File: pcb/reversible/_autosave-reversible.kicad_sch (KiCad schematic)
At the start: 83 parts, among them J1 PJ-320A, P1 OLED, SW1 Kailh hotswap MX socket, SW10 Kailh hotswap MX socket, SW11 Kailh hotswap MX socket, SW12 Kailh hotswap MX socket, SW13 Kailh hotswap MX socket, SW14 Kailh hotswap MX socket, SW15 Kailh hotswap MX socket, SW16 Kailh hotswap MX socket, SW17 Kailh hotswap MX socket, SW18 Kailh hotswap MX socket, SW19 Kailh hotswap MX socket, SW2 Kailh hotswap MX socket, SW20 Kailh hotswap MX socket, SW21 Kailh hotswap MX socket, SW22 Kailh hotswap MX socket, SW23 Kailh hotswap MX socket, SW24 Kailh hotswap MX socket, SW25 Kailh hotswap MX socket, SW26 Kailh hotswap MX socket, SW27 Kailh hotswap MX socket, SW28 Kailh hotswap MX socket, SW29 Kailh hotswap MX socket, SW3 Kailh hotswap MX socket, SW4 Kailh hotswap MX socket, SW5 Kailh hotswap MX socket, SW6 Kailh hotswap MX socket, SW7 Kailh hotswap MX socket, SW8 Kailh hotswap MX socket, SW9 Kailh hotswap MX socket, U1 ProMicro

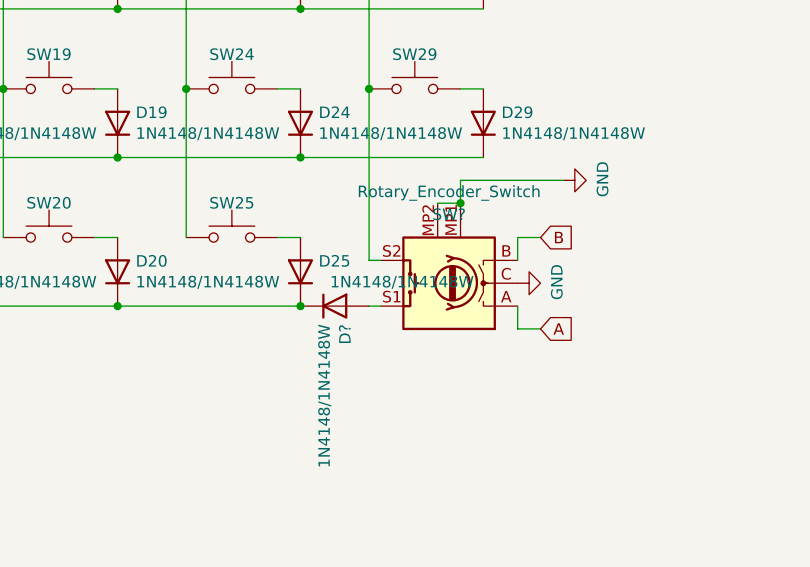
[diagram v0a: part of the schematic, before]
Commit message: layout designed
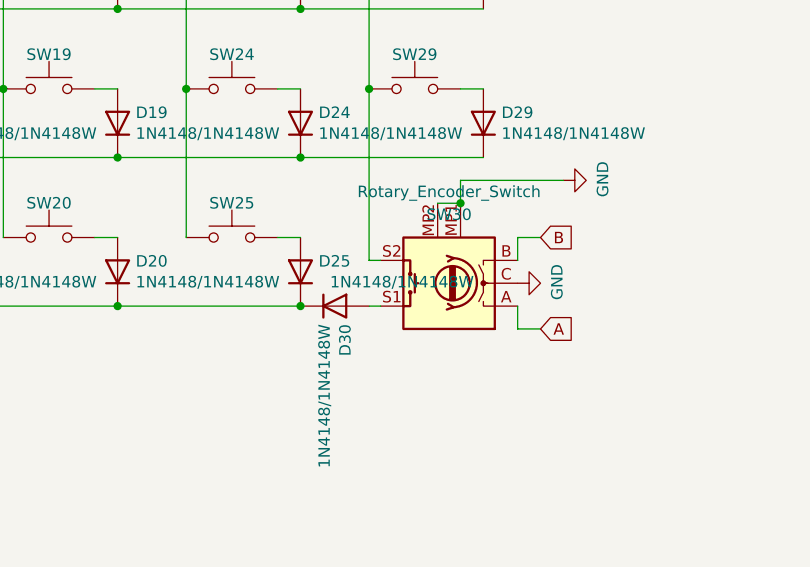
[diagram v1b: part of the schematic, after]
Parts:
- D30: renamed from D?; footprint Keyboard Library:Diode_DO35_SOD123 -> lowProfile:Diode_TH_SOD123
- SW30: renamed from SW?; footprint Keyboard Library:RotaryEncoder_Alps_EC11E-Switch_Vertical_H20_special -> lowProfile:RotaryEncoder_Alps_EC12E-Switch_Vertical_H20mm
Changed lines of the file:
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@@
 		(on_board yes)
 		(dnp no)
-		(property "Reference" "SW?"
+		(property "Reference" "SW30"
 			(at 139.7 97.79 0)
 			(effects
@@
 			)
 		)
-		(property "Footprint" "Keyboard Library:RotaryEncoder_Alps_EC11E-Switch_Vertical_H20_special"
+		(property "Footprint" "lowProfile:RotaryEncoder_Alps_EC12E-Switch_Vertical_H20mm"
 			(at 143.51 109.474 0)
 			(effects
@@
 			(project "reversible"
 				(path "/4b5512f1-4036-44b1-a4c2-dbd3b8563587"
-					(reference "SW?")
+					(reference "SW30")
 					(unit 1)
 				)
@@
 		(on_board yes)
 		(dnp no)
-		(property "Reference" "D?"
+		(property "Reference" "D30"
 			(at 128.1684 109.9566 90)
 			(effects
@@
 			)
 		)
-		(property "Footprint" "Keyboard Library:Diode_DO35_SOD123"
+		(property "Footprint" "lowProfile:Diode_TH_SOD123"
 			(at 127 107.95 0)
 			(effects
@@
 			(project "reversible"
 				(path "/4b5512f1-4036-44b1-a4c2-dbd3b8563587"
-					(reference "D?")
+					(reference "D30")
 					(unit 1)
 				)
